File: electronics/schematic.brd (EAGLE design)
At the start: 20.3 x 15.9 mm, 22 parts, among them Q2 NX3008NBK

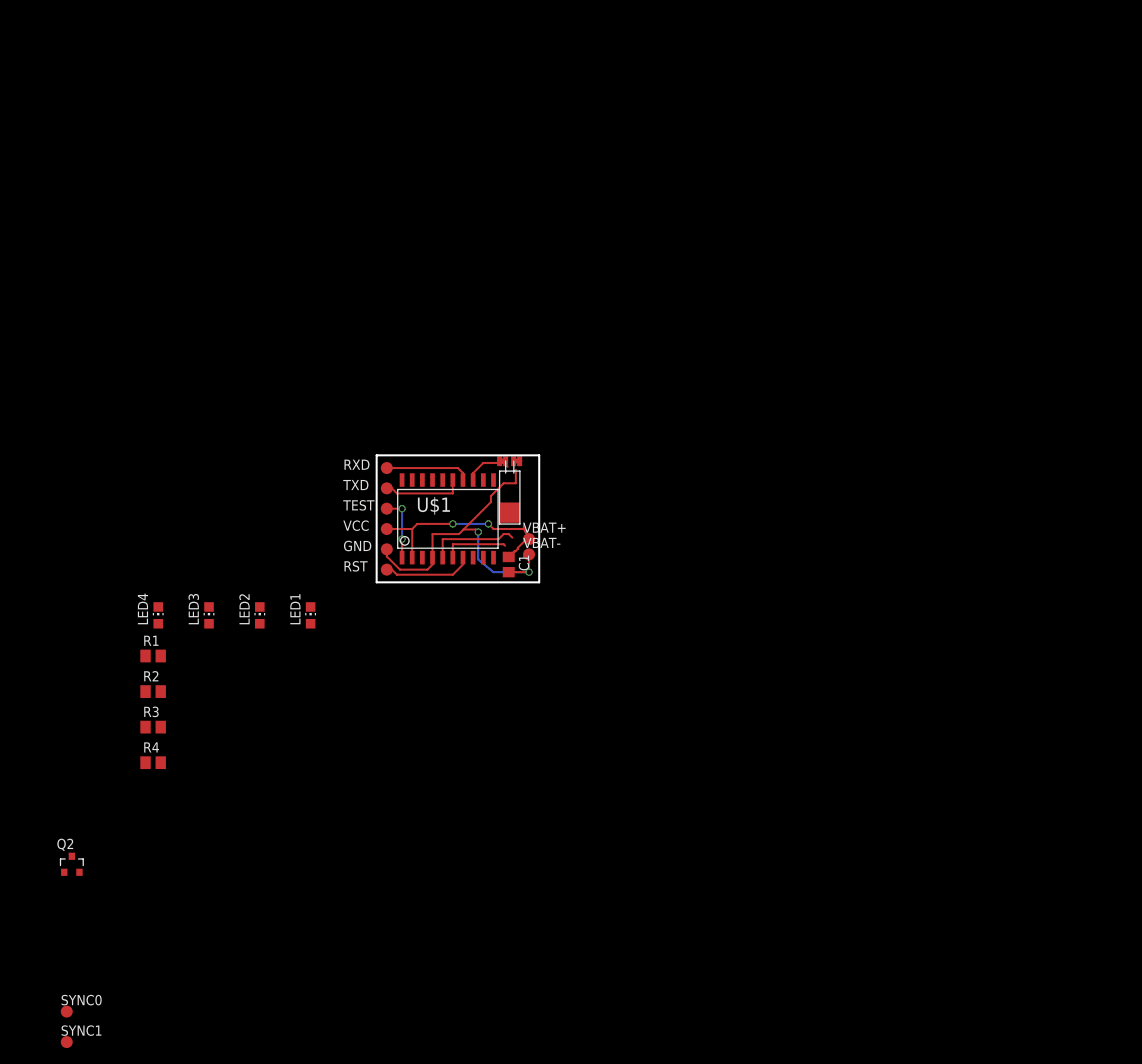
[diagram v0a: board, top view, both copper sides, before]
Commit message: new board design
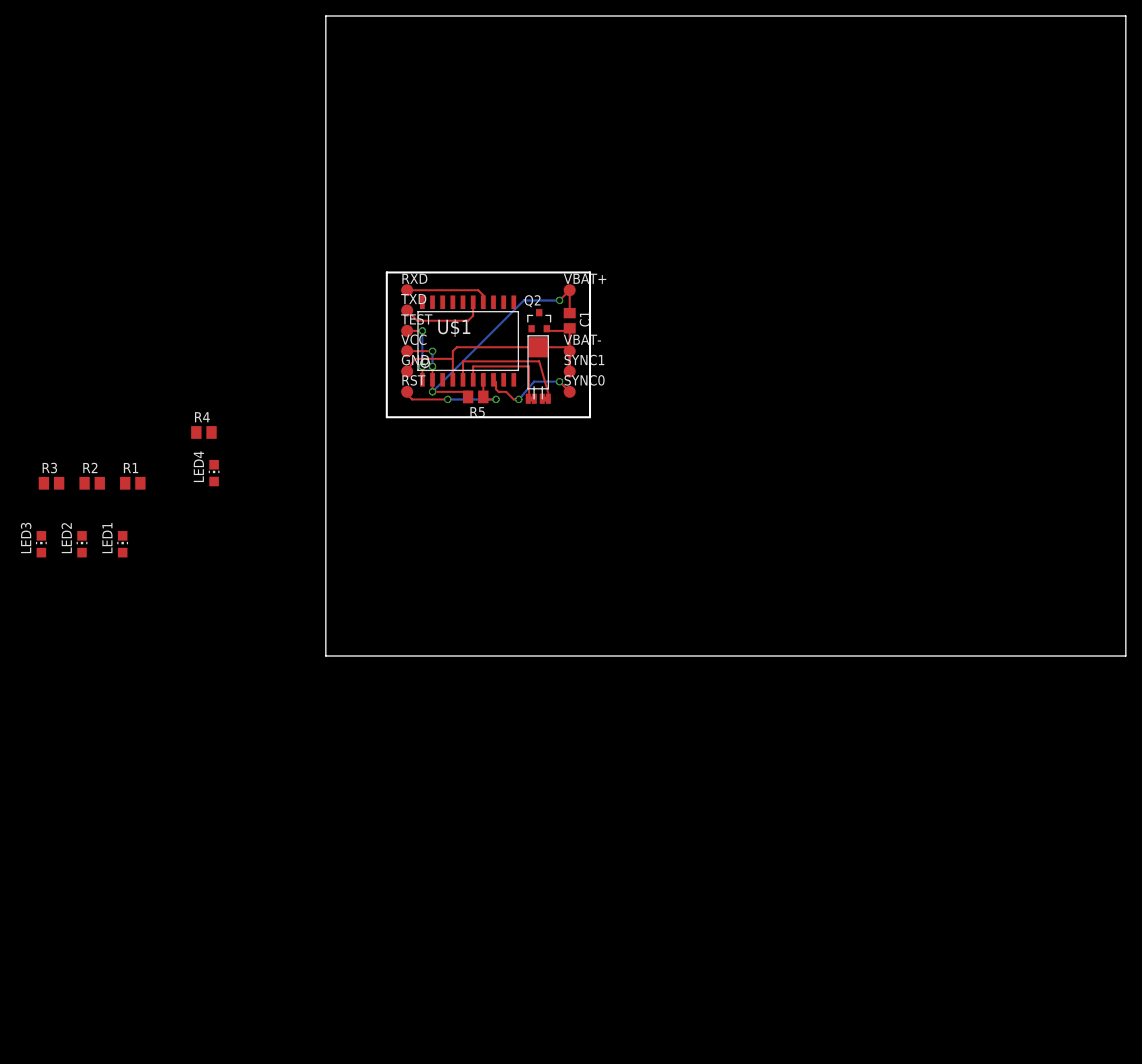
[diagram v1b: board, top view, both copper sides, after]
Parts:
- added R5: (no value), resistor:M0805
- moved SYNC1 104.8 mm to (30.5, 35.6)
- moved SYNC0 99.8 mm to (30.5, 33.0)
- moved Q2 89.6 mm to (26.7, 41.9)
- moved R4 41.8 mm to (-15.2, 27.9)
- moved R3 33.0 mm to (-34.3, 21.6)
- moved VBAT+ 31.5 mm to (30.5, 45.7)
- moved C1 31.4 mm to (30.5, 41.9)
- moved R2 27.1 mm to (-29.2, 21.6)
- moved VBAT- 25.9 mm to (30.5, 38.1)
- moved LED1 25.1 mm to (-25.4, 14.0)
- moved LED2 23.9 mm to (-30.5, 14.0)
- moved LED3 22.8 mm to (-35.6, 14.0)
- moved GND 22.4 mm to (10.2, 35.6)
- moved RST 22.4 mm to (10.2, 33.0)
- moved TEST 22.4 mm to (10.2, 40.6)
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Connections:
- net LED: no longer U$1.13
- net RST: now also R5.1, U$1.7
- net VCC: now also R5.2; no longer U$1.7
- net XIN: now also U$2.P$2; no longer U$2.P$1
- net XOUT: now also U$2.P$1; no longer U$2.P$2
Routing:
- net P2.0: track 0.00 -> 12.6 mm, vias 0 -> 2
- net VCC: track 27.5 -> 38.6 mm, vias 2 -> 4
- net GND: track 44.4 -> 36.4 mm, vias 2 -> 0
- net LED: track 5.89 -> 0.00 mm
- net RST: track 10.3 -> 15.6 mm, vias 0 -> 2
- net XOUT: track 11.5 -> 16.5 mm
- net XIN: track 8.29 -> 12.5 mm
- net TXD: track 10.2 -> 10.7 mm
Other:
- board size 20.3 x 15.9 mm -> 100 x 80 mm
